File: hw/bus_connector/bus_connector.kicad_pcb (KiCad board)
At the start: 2 copper layers, 68.7 x 35.4 mm, 11 parts, among them J1 DB9_Top, J2 DB9_Left, J3 DB9_Right

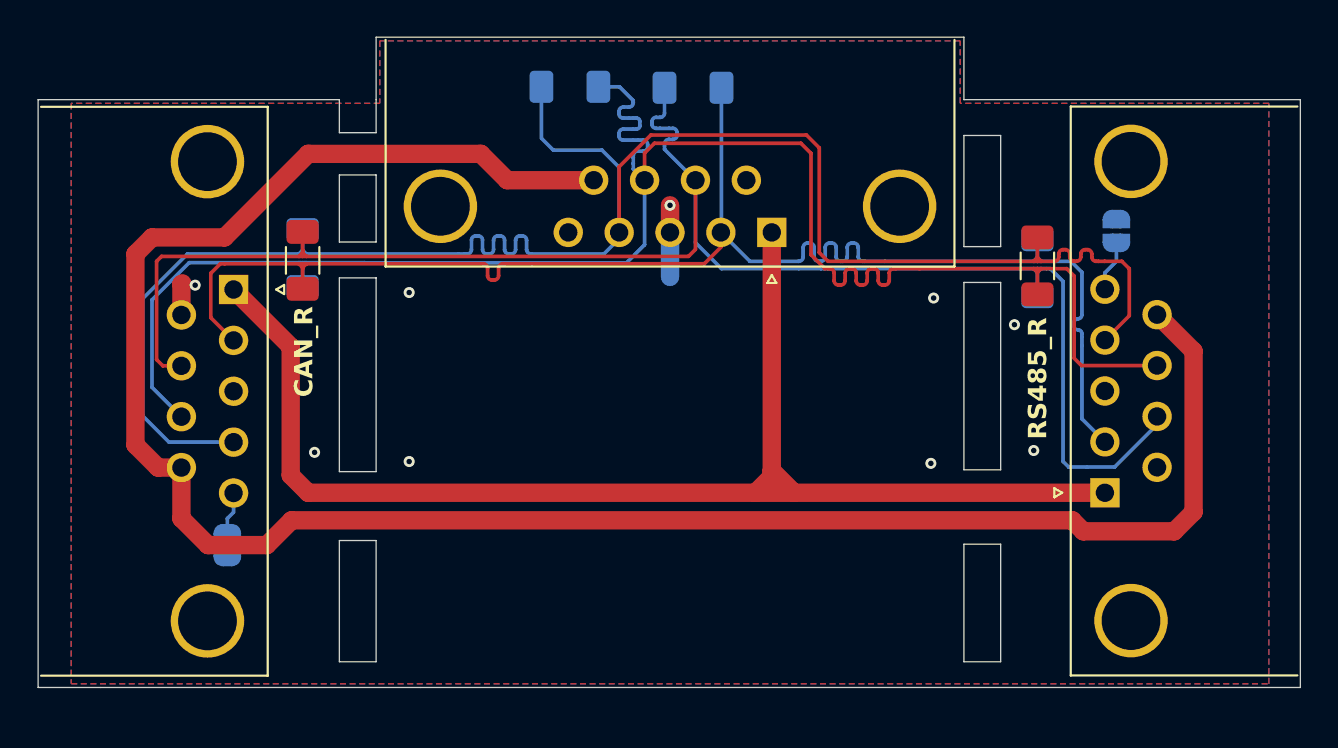
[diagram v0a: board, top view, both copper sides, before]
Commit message: Edit actions
Signed-off-by: Mateusz Pająk <22417805+Tai-Min@users.noreply.github.com>
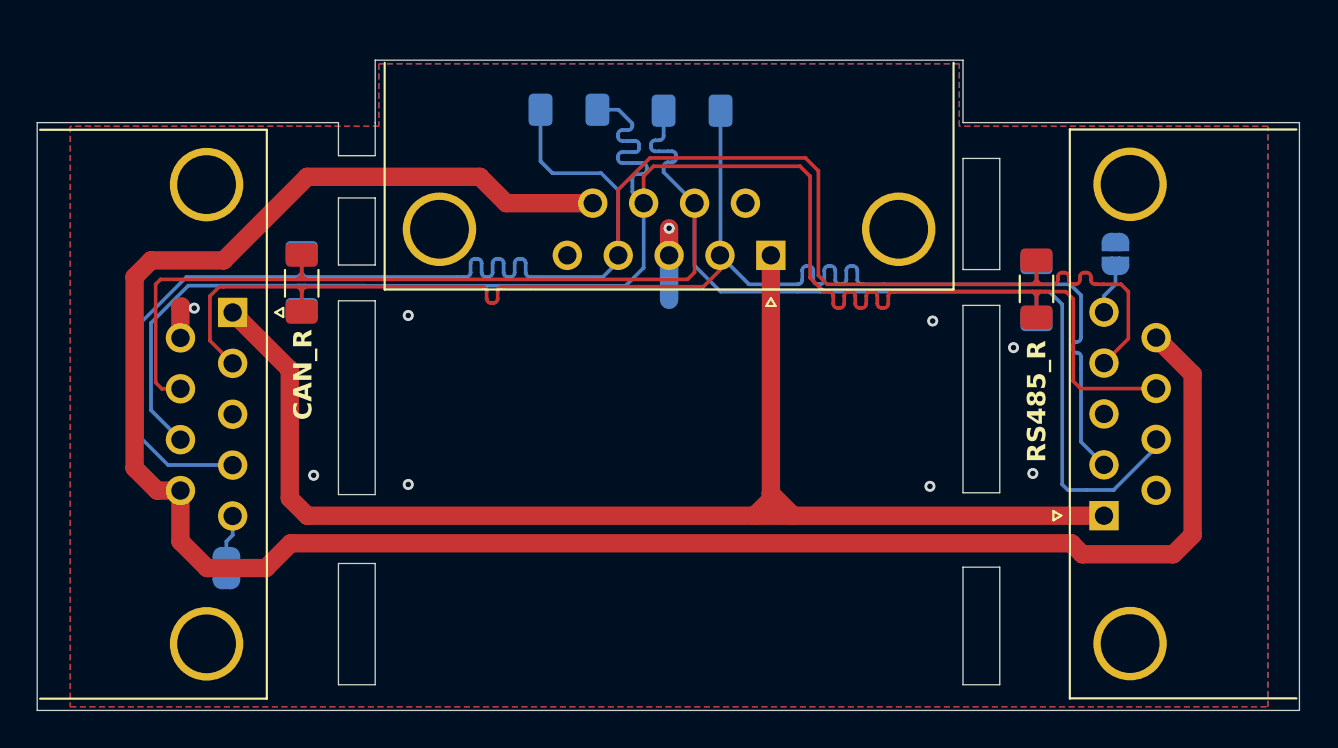
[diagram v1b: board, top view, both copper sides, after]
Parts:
- moved JP1 1.25 mm to (170.8, 100.0)
- moved R1 1.25 mm to (141.1, 92.2)
- moved J3 1.25 mm to (122.8, 103.2)
- moved JP3 1.25 mm to (122.5, 117.1)
- moved R3 1.25 mm to (126.5, 101.5)
- moved R4 1.25 mm to (126.5, 101.6)
- moved J1 1.25 mm to (152.1, 100.1)
- moved J2 1.25 mm to (170.2, 114.2)
- moved R2 1.25 mm to (147.8, 92.2)
- moved R5 1.25 mm to (166.6, 101.9)
- moved R6 1.25 mm to (166.6, 102.0)

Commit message: Fix issues with bus connector project
Signed-off-by: Mateusz Pająk <22417805+Tai-Min@users.noreply.github.com>
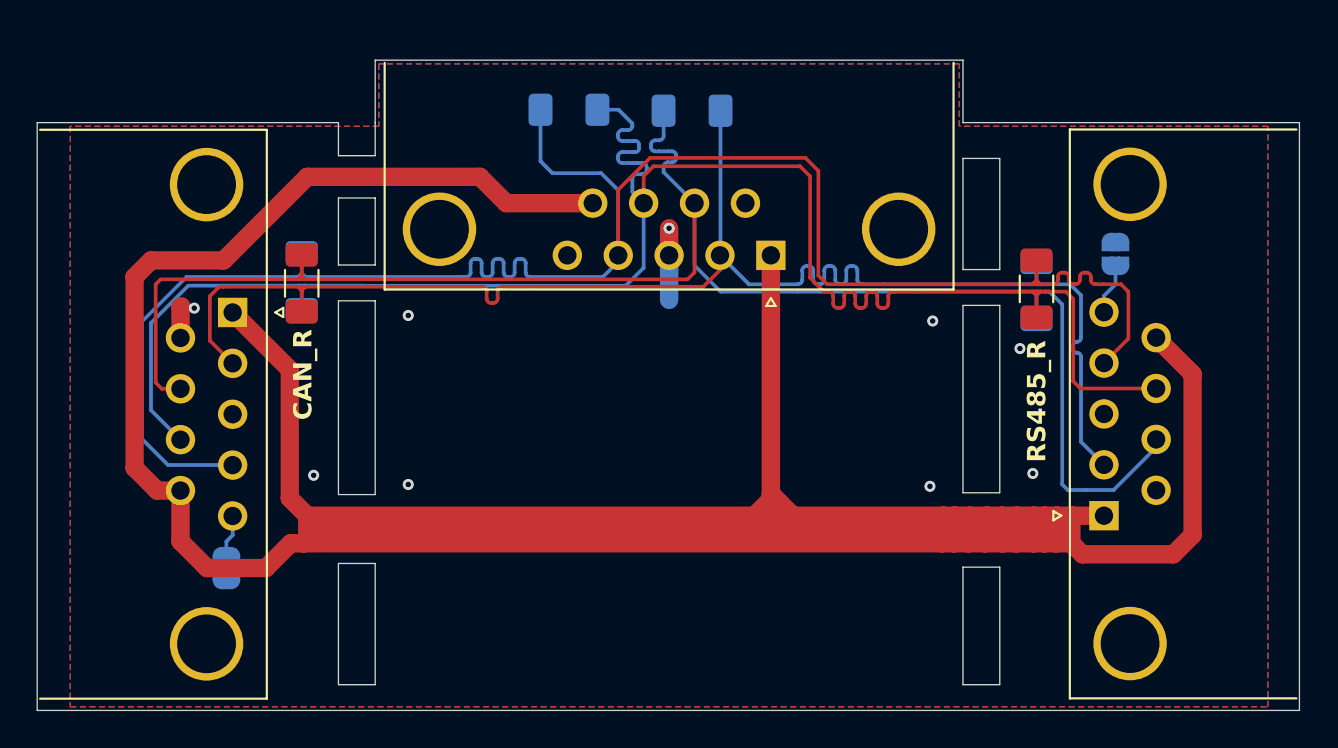
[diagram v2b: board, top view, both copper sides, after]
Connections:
- J1 pad 5: SHIELD -> unconnected-(J1-Pad5)
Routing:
- net VCC: track 184.9 -> 236.7 mm
